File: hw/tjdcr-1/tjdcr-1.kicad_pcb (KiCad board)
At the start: 4 copper layers, 100 x 35 mm, 72 parts, among them J1 Conn_Coaxial, J2 Tuning, J3 Power, J4 LO Option, J5 Volume, J6 Speaker, Q1 MMBT3904, Q2 MMBFJ310, Q3 MMBT3904, Q4 MMBT3904, Q5 2N3904, T1 5:28, T2 28:5, T3 Transformer_1P_2S, T4 Transformer_1P_2S, T5 42TL013-RC

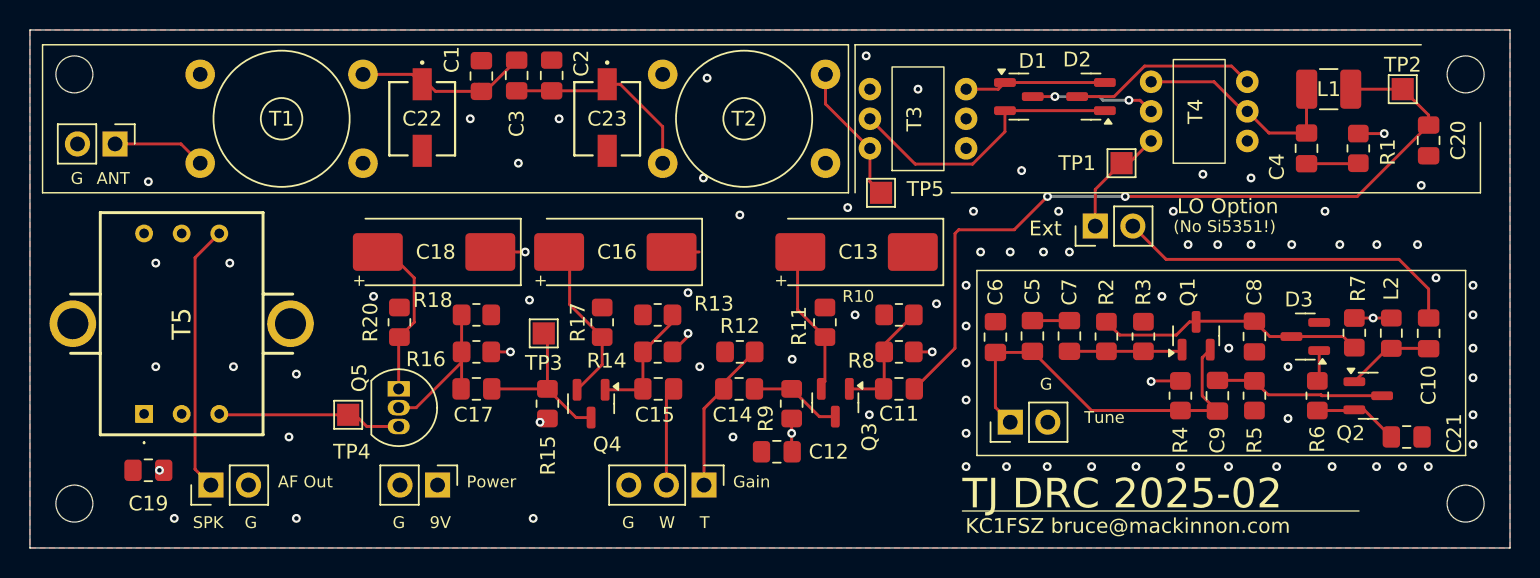
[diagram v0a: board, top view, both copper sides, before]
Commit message: Ready to send this version to fab
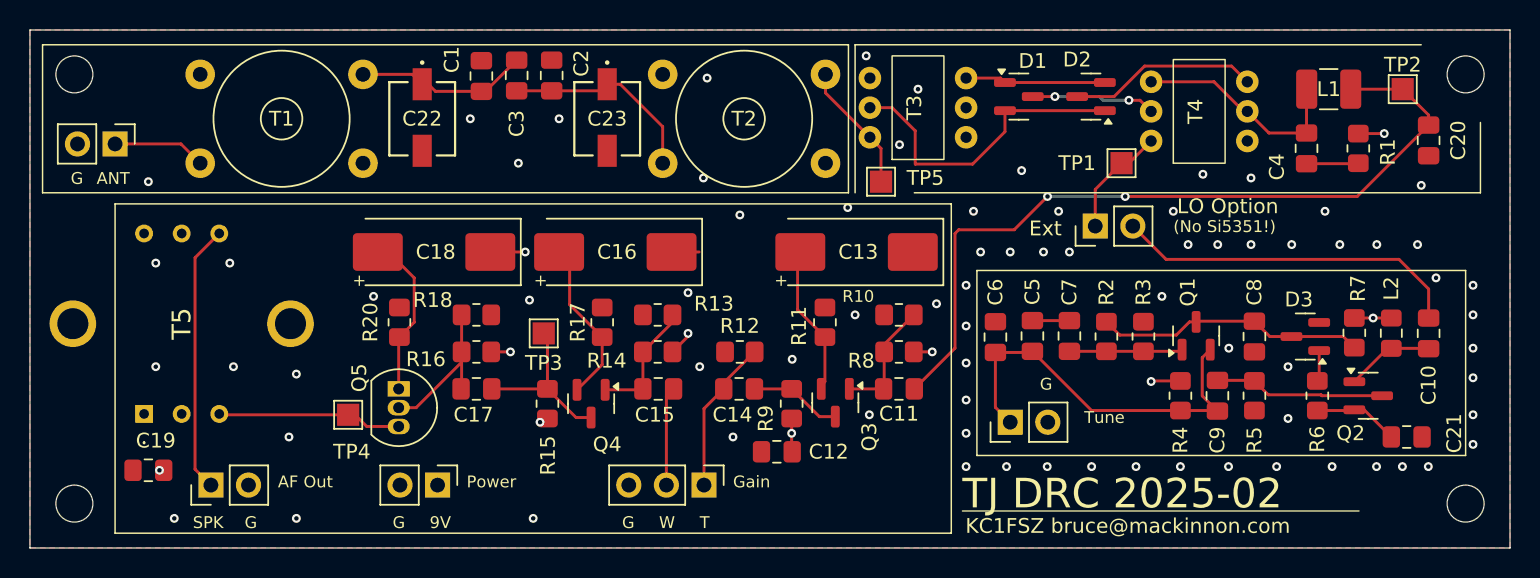
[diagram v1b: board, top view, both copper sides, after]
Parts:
- C1, C2: value 160p -> 150p
- moved T3 0.75 mm to (133.8, 56.2)
- moved TP5 0.75 mm to (131.5, 61.2)
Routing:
- net Net-(D1-K): track 19.5 -> 21.1 mm
- net Net-(T1-SB): track 13.2 -> 11.7 mm
- net Net-(T2-SB): track 14.5 -> 13.7 mm
- net Net-(T2-AA): track 9.55 -> 8.80 mm
- net GND: vias 78 -> 79
